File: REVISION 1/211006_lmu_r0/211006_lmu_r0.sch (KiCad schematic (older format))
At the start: 4 parts

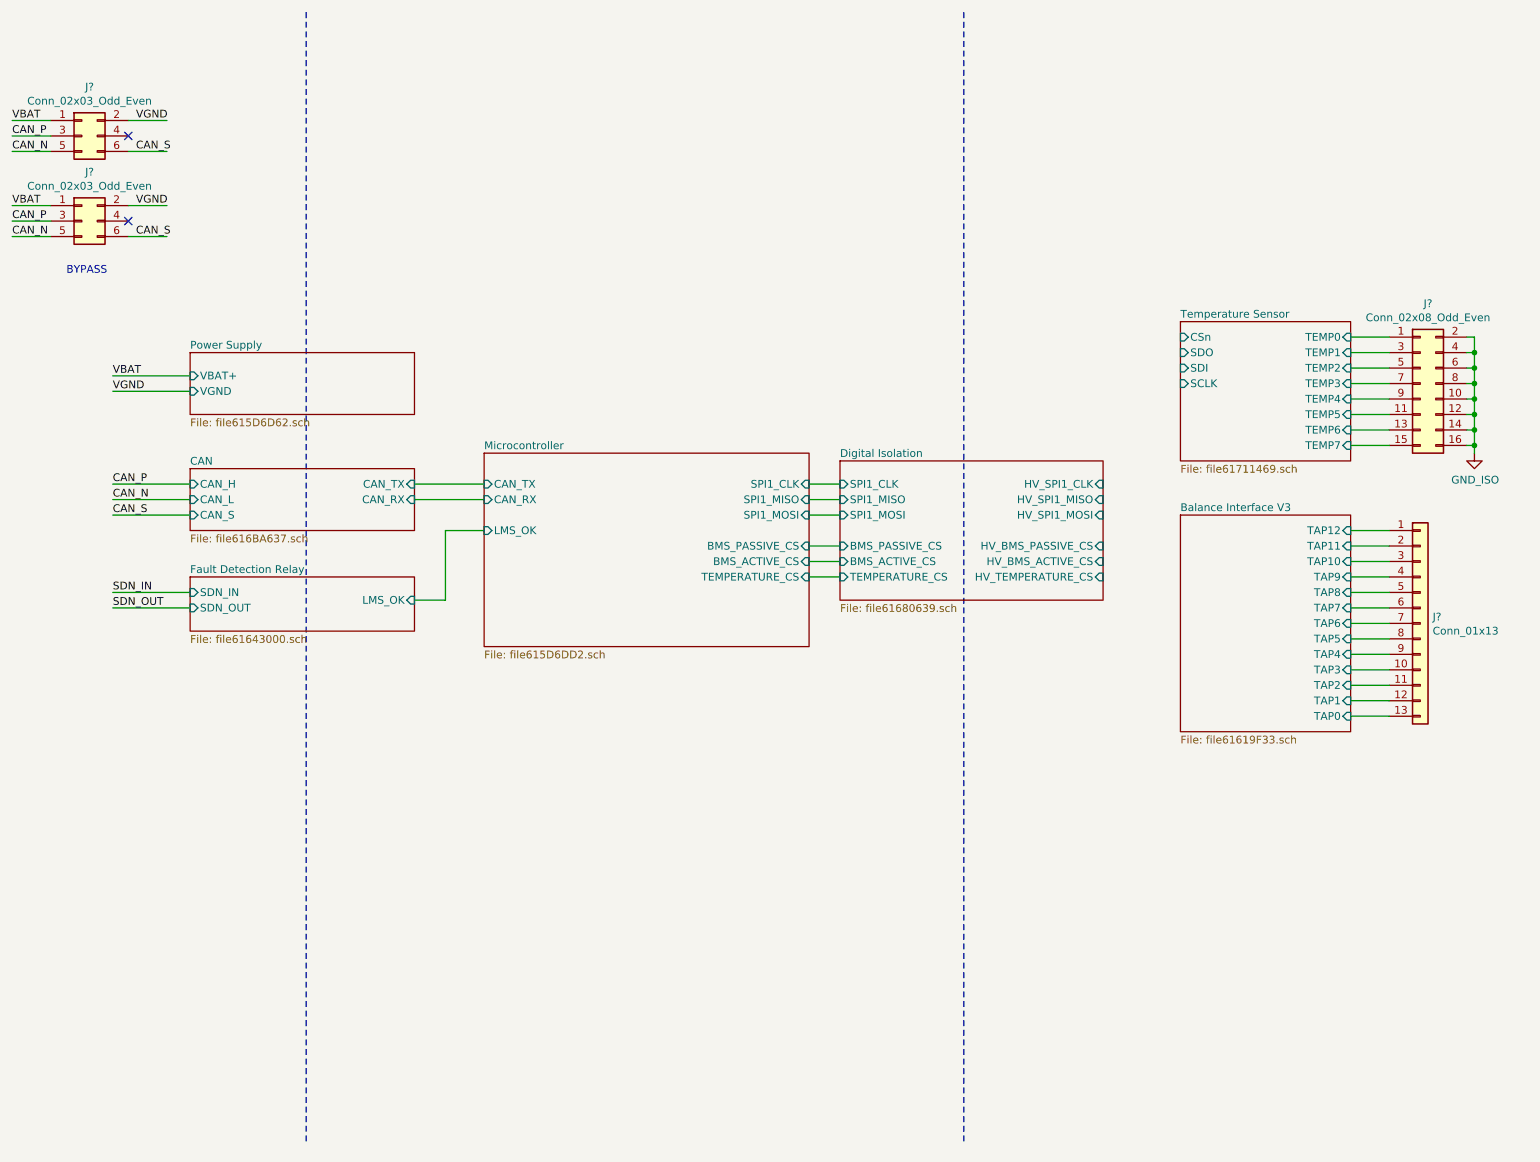
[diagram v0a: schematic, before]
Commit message: Finished schematic, ready for pcb layout
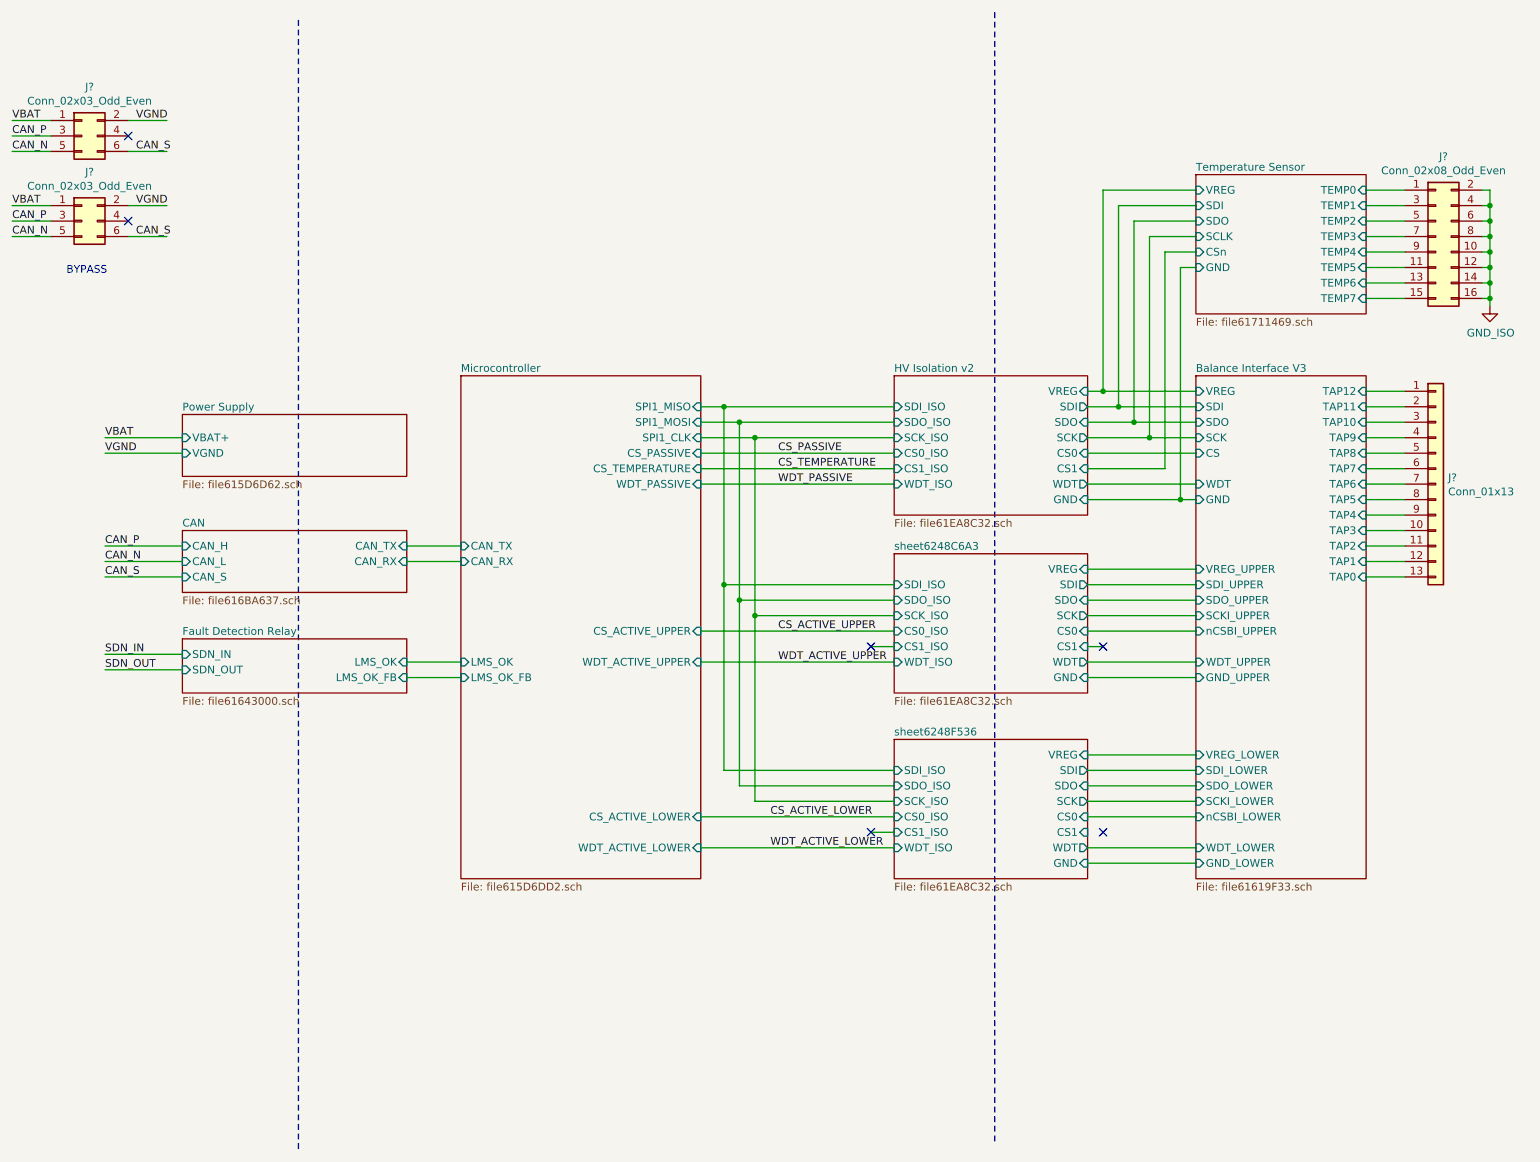
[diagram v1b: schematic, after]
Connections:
- net labels added: CS_ACTIVE_LOWER, CS_ACTIVE_UPPER, CS_PASSIVE, CS_TEMPERATURE, WDT_ACTIVE_LOWER, WDT_ACTIVE_UPPER, WDT_PASSIVE
- wire segments 65 -> 125
- no-connect marks 2 -> 6
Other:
- moved on the sheet: J?
